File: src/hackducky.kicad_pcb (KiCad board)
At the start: 2 copper layers, 21 x 47 mm, 51 parts, among them J1 USB_A, J2 Conn_02x02_Top_Bottom, J3 Micro_SD_Card, P2 USB_C_Plug, SW3 BOOT_SEL, SW4 BOOT_SEL, U1 W25Q16JVSS, U2 AP2112K-3.3, U3 USBLC6-2P6, U4 RP2040, U5 USBLC6-2P6, Y1 Crystal_GND24

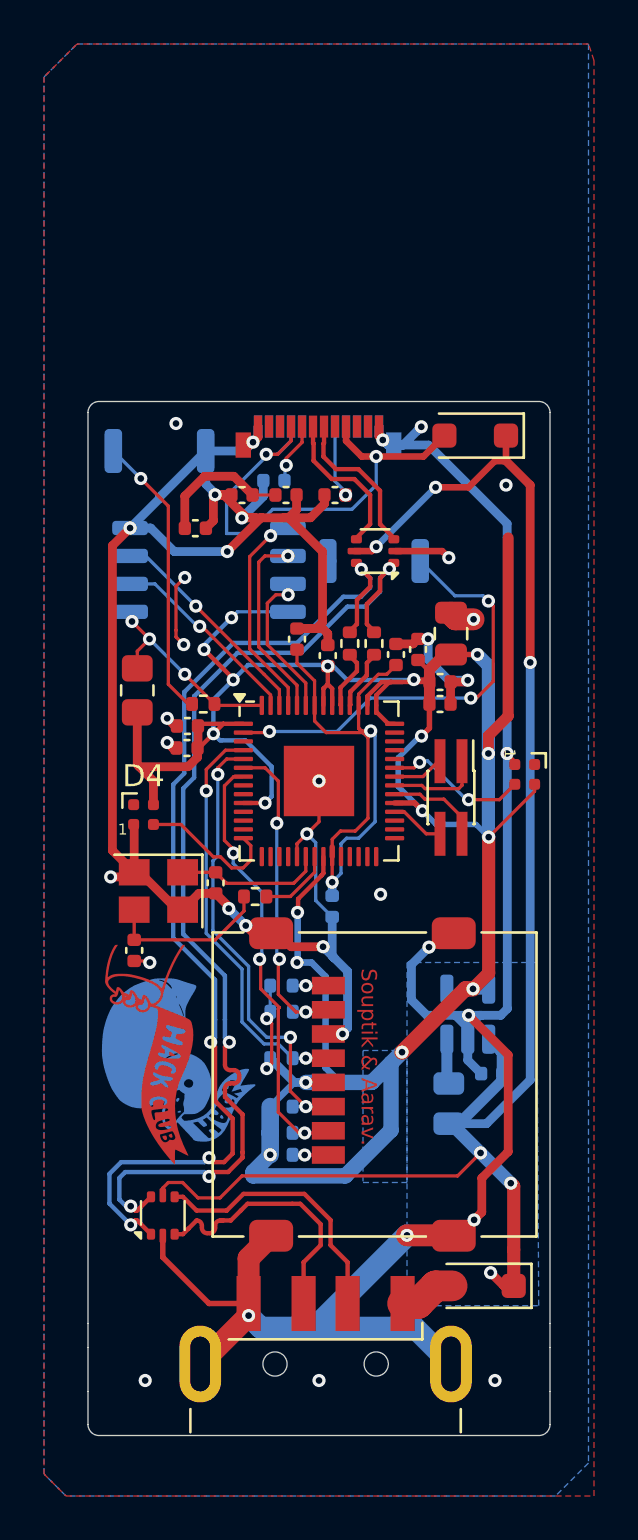
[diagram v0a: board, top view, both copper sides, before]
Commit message: new sm fic
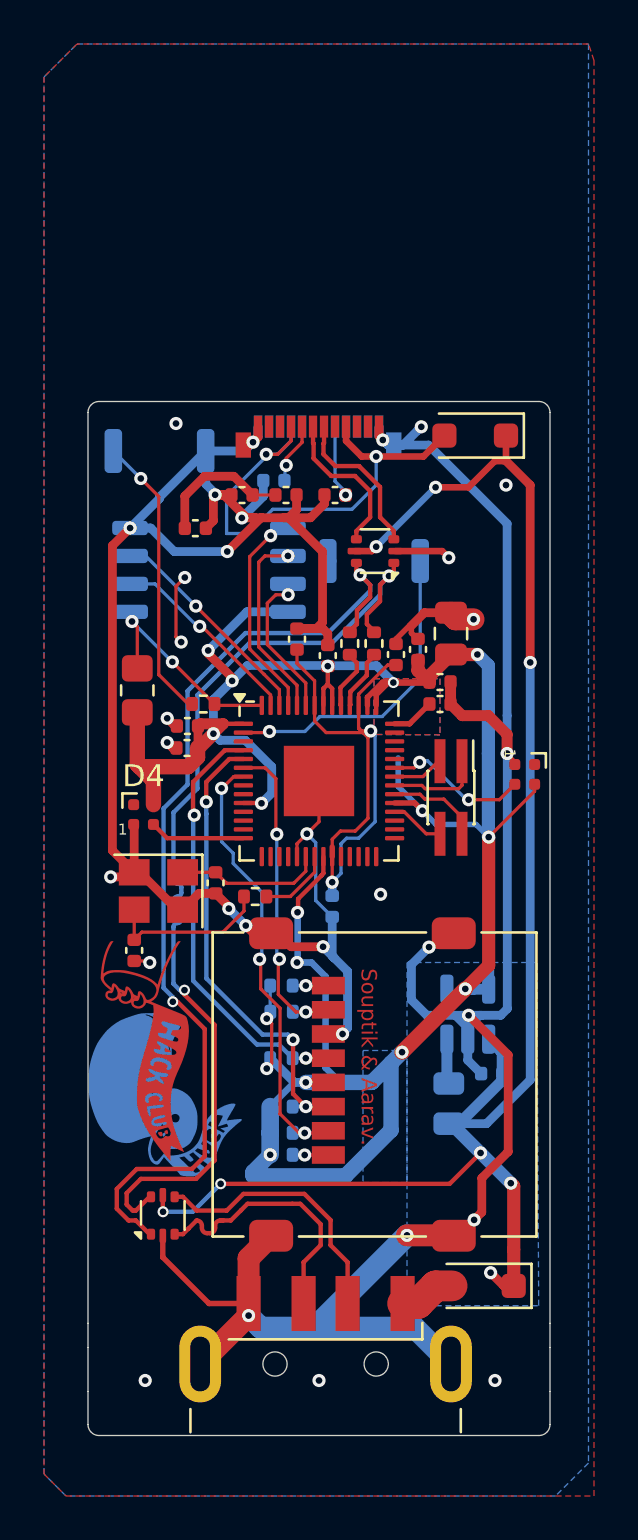
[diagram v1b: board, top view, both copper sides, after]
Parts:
- moved G*** 1.70 mm to (82.7, 95.0) (x2)
- moved G*** 0.26 mm to (82.1, 93.0)
- moved G*** 0.25 mm to (82.1, 93.0)
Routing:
- net +3V3: track 154.5 -> 138.2 mm, vias 23 -> 20
- net GPIO0: track 19.9 -> 14.4 mm, vias 3 -> 1
- net D-: track 47.8 -> 44.9 mm, vias 4 -> 2
- net D+: track 47.8 -> 44.9 mm, vias 4 -> 2
- net GND: track 189.5 -> 191.8 mm, vias 32 -> 29
- net GPIO11: track 6.53 -> 4.35 mm
- net SD_CLK: track 18.8 -> 19.6 mm
- net QSPI_SS: track 9.80 -> 10.5 mm, vias 3 -> 2
- net +5V: track 74.1 -> 74.4 mm, vias 6 -> 8
- added copper zone on B.Cu, net +3V3
